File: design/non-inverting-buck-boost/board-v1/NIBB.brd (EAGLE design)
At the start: 100 x 54.6 mm, 13 parts

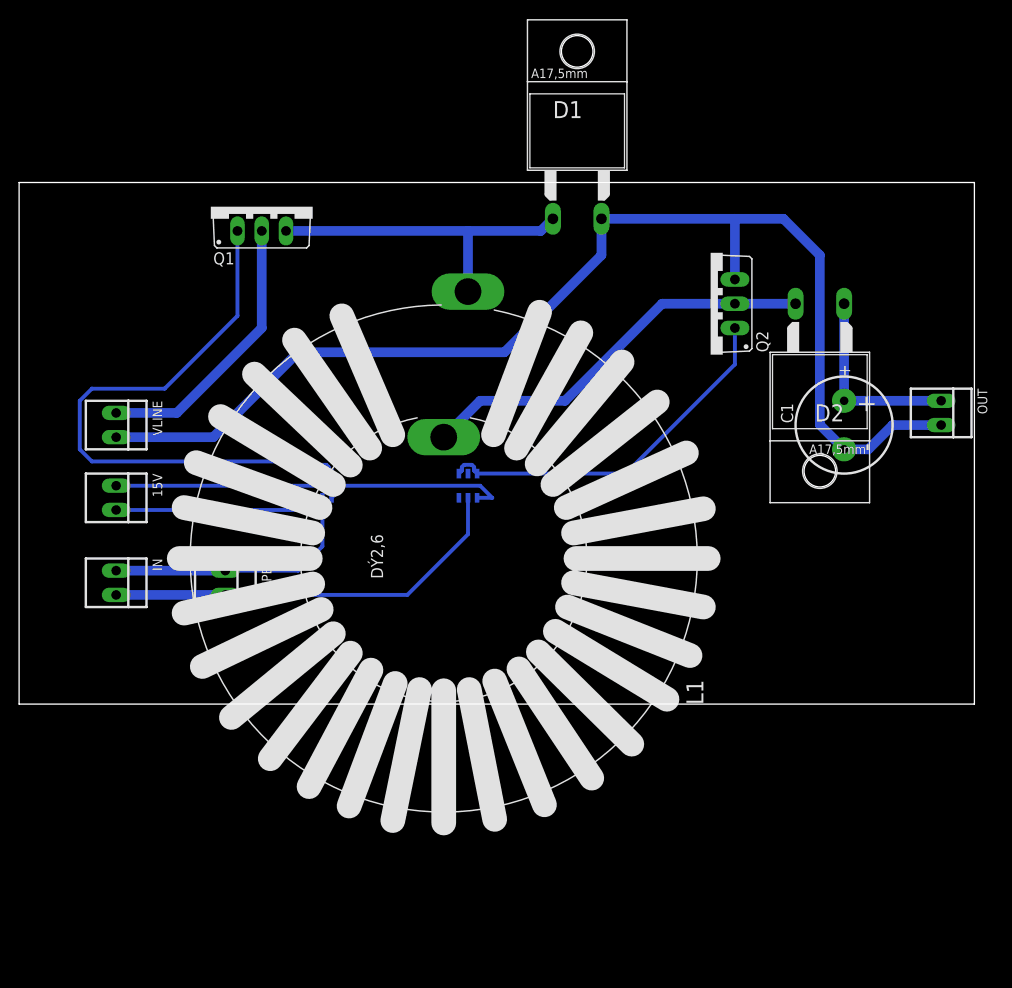
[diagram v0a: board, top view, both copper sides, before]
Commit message: finished v1 layout
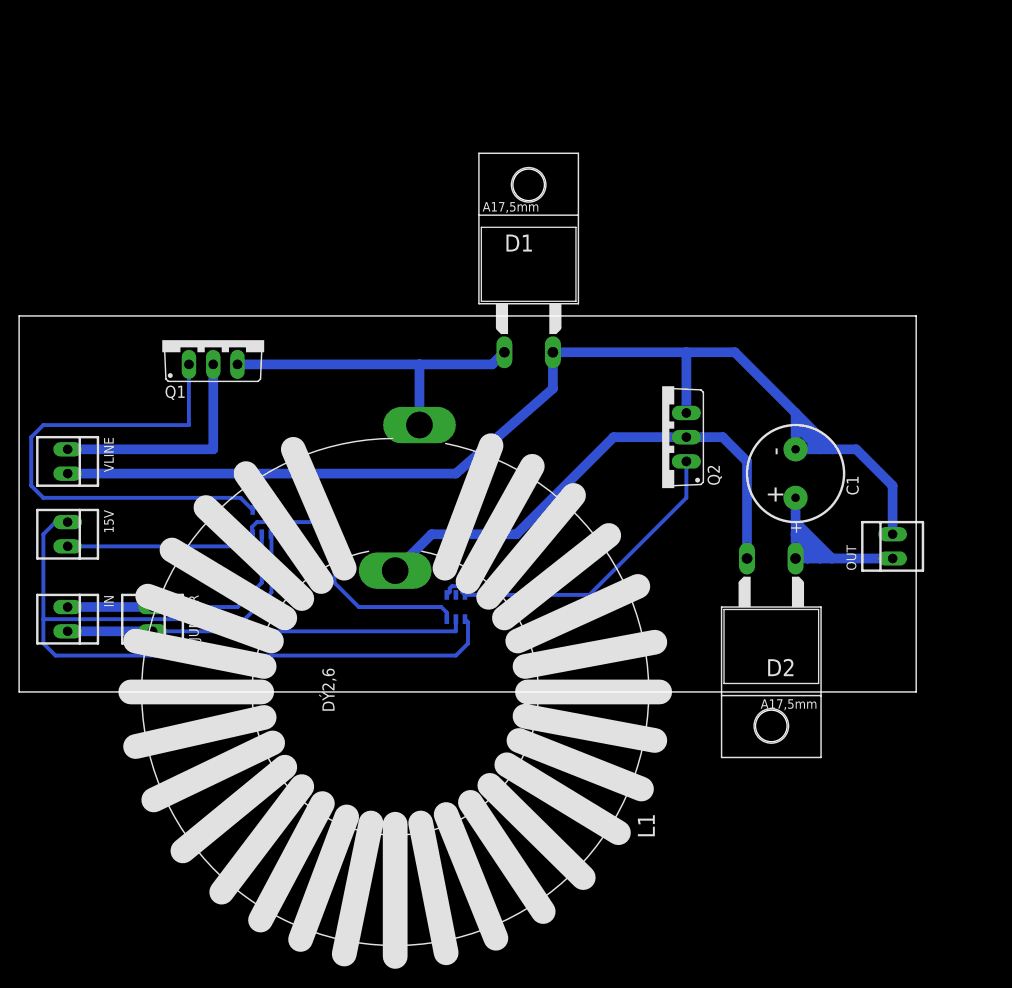
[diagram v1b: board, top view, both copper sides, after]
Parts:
- moved D2 27.1 mm to (78.7, 7.62)
- moved D1 14.9 mm to (53.3, 41.9)
- moved L1 14.9 mm to (39.4, 0.00)
- moved OUT 14.9 mm to (91.4, 15.2), turned to 90 degrees
- moved Q1 14.9 mm to (20.3, 36.8)
- moved Q2 14.9 mm to (67.3, 26.7)
- moved IC2 12.8 mm to (45.7, 8.89)
- moved JUMPER 8.52 mm to (14.0, 7.62)
- moved IC1 7.41 mm to (25.4, 17.8)
- moved C1 7.18 mm to (81.3, 22.9), turned to 90 degrees
- moved VLINE 6.35 mm to (5.08, 24.1)
- moved IN 6.35 mm to (5.08, 7.62)
- moved 15V 6.35 mm to (5.08, 16.5)
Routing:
- net 15V+: track 42.9 -> 93.8 mm
- net 15V-: track 21.2 -> 48.9 mm
- net N$2: track 42.6 -> 53.8 mm
- net N$7: track 20.3 -> 27.3 mm
- net N$5: track 62.8 -> 55.8 mm
- net N$3: track 29.1 -> 24.1 mm
- net N$6: track 38.6 -> 34.3 mm
- net N$4: track 125.9 -> 121.9 mm
- net IN2: track 43.3 -> 41.9 mm
- net IN1: track 27.7 -> 26.5 mm
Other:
- board size 100 x 54.6 mm -> 93.9 x 39.4 mm
